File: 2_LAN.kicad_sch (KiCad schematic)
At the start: 48 parts, among them U1 LAN9514, X1 25MHz

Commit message: add LCSC part tags, silkscreen
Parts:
- C10, C9: LCSC (none) -> C1658
- C11: LCSC (none) -> C1779
- C12, C13, C14, C15, C16, C17, C18, C21, C22, C23, C24, C25, C26, C27, C28: LCSC (none) -> C14663
- C19: LCSC (none) -> C21122
- C29: LCSC (none) -> C1592
- C45, C46: LCSC (none) -> C23742
- D1: LCSC (none) -> C2687126
- F2: LCSC (none) -> C2830246
- FB1, FB2: LCSC (none) -> C14709
- LAN1: LCSC (none) -> C3021374
- R10, R12: LCSC (none) -> C25804
- R11: LCSC (none) -> C22790
- R13, R9: LCSC (none) -> C23138
- R21, R22, R23, R24, R25, R26, R27, R30: LCSC (none) -> C21189
- R6: LCSC (none) -> C22935
- R7: LCSC (none) -> C22865
- R8: LCSC (none) -> C22859
- RN1: LCSC (none) -> C136850
- U1: LCSC (none) -> C625111
- USB1, USB2: LCSC (none) -> C6386909
- X1: LCSC (none) -> C9006

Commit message: rename to x1-expander
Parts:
- C10, C9: symbol X1 Expande-easyedapro:33pF -> x1-expander:33pF
- C11: symbol X1 Expande-easyedapro:4.7uF -> x1-expander:4.7uF
- C12, C13, C14, C15, C16, C17, C18, C21, C22, C23, C24, C25, C26, C27, C28: symbol X1 Expande-easyedapro:100nF -> x1-expander:100nF
- C19: symbol X1 Expande-easyedapro:.022uF -> x1-expander:.022uF
- C29: symbol X1 Expande-easyedapro:1uF -> x1-expander:1uF
- C45, C46: symbol X1 Expande-easyedapro:75pF -> x1-expander:75pF
- D1: footprint X1 Expande-easyedapro:SOT-23-6_L2.9-W1.6-P0.95-LS2.8-BL -> x1-expander:SOT-23-6_L2.9-W1.6-P0.95-LS2.8-BL; symbol X1 Expande-easyedapro:SRV05-4.TCT_C2687126 -> x1-expander:SRV05-4.TCT_C2687126
- F2: symbol X1 Expande-easyedapro:JK-NSMD100-16V -> x1-expander:JK-NSMD100-16V
- FB1, FB2: symbol X1 Expande-easyedapro:2A/0.05DCR -> x1-expander:2A/0.05DCR
- LAN1: footprint X1 Expande-easyedapro:RJ45-TH_HC913550A-M899-A -> x1-expander:RJ45-TH_HC913550A-M899-A; symbol X1 Expande-easyedapro:HC913550A-M899-A -> x1-expander:HC913550A-M899-A
- R10, R12: symbol X1 Expande-easyedapro:10K 1/10W 1% -> x1-expander:10K 1/10W 1%
- R11: symbol X1 Expande-easyedapro:12k 1/10W 1% -> x1-expander:12k 1/10W 1%
- R13, R9: symbol X1 Expande-easyedapro:330 -> x1-expander:330
- R6: symbol X1 Expande-easyedapro:1M -> x1-expander:1M
- R7: symbol X1 Expande-easyedapro:12.4k 1% -> x1-expander:12.4k 1%
- R8: symbol X1 Expande-easyedapro:10 1/16W 1% -> x1-expander:10 1/16W 1%
- RN1: footprint X1 Expande-easyedapro:RES-ARRAY-SMD_0402-8P-L2.0-W1.0-BL -> x1-expander:RES-ARRAY-SMD_0402-8P-L2.0-W1.0-BL; symbol X1 Expande-easyedapro:49.9 -> x1-expander:49.9
- U1: footprint X1 Expande-easyedapro:QFN64G-0.5-9X9MM -> x1-expander:QFN64G-0.5-9X9MM; symbol X1 Expande-easyedapro:LAN9514 -> x1-expander:LAN9514
- USB1, USB2: footprint X1 Expande-easyedapro:USB-TH_10.0-4C6.3-ZB -> x1-expander:USB-TH_10.0-4C6.3-ZB; symbol X1 Expande-easyedapro:10.0 4C6.3 ZB -> x1-expander:10.0 4C6.3 ZB
- X1: footprint X1 Expande-easyedapro:OSC-SMD_4P-L3.2-W2.5-BL -> x1-expander:OSC-SMD_4P-L3.2-W2.5-BL; symbol X1 Expande-easyedapro:25MHz -> x1-expander:25MHz

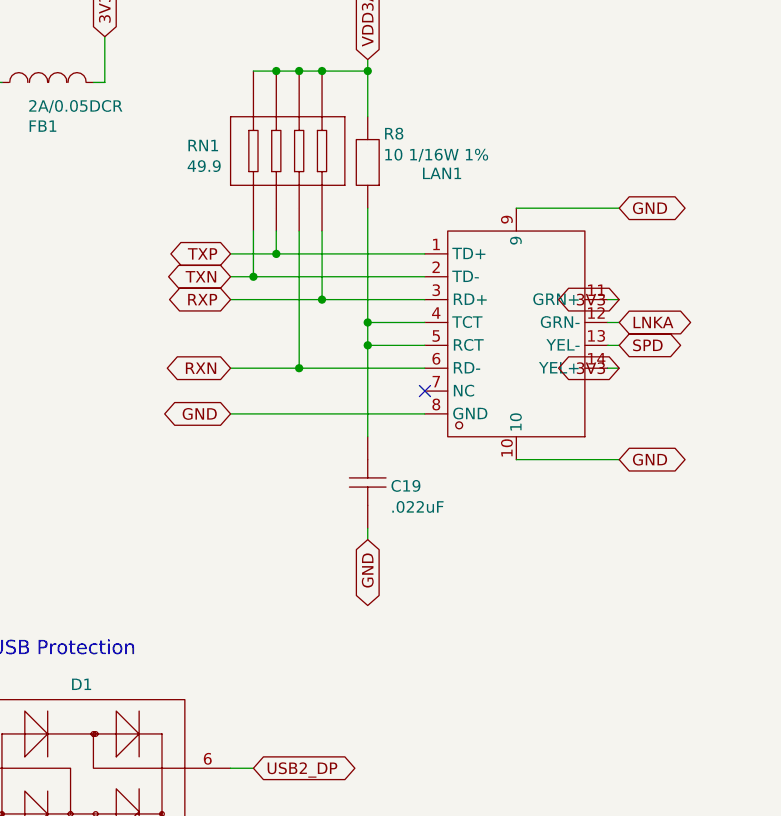
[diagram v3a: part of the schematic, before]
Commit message: replace LAN1 with C375844
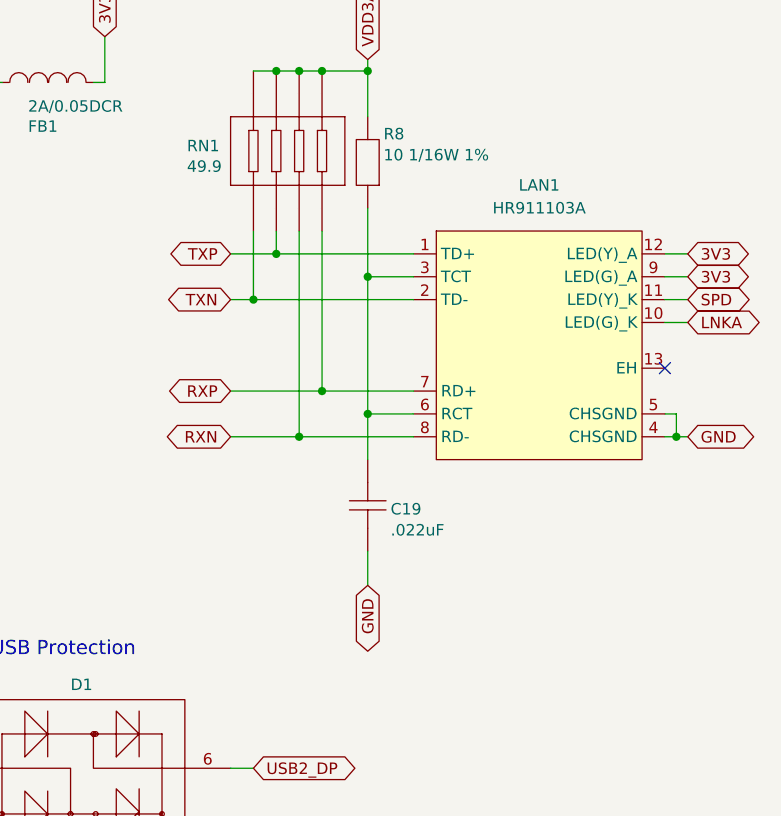
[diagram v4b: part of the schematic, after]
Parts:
- removed LAN1: HC913550A-M899-A, x1-expander:RJ45-TH_HC913550A-M899-A, symbol x1-expander:HC913550A-M899-A
- added LAN1: HR911103A, x1-expander:RJ45-TH_HR911103A, symbol x1-expander:HR911103A
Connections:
- net 3V3: now also LAN1.12 (LED(Y)_A), LAN1.9 (LED(G)_A)
- net GND: now also LAN1.4 (CHSGND), LAN1.5 (CHSGND)
- net LNKA: now also LAN1.10 (LED(G)_K)
- net RXN: now also LAN1.8 (RD-)
- net RXP: now also LAN1.7 (RD+)
- net SPD: now also LAN1.11 (LED(Y)_K)
- net TXN: now also LAN1.2 (TD-)
- net TXP: now also LAN1.1 (TD+)
- net at C19.2, R8.1: now also LAN1.3 (TCT), LAN1.6 (RCT)
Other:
- moved on the sheet: C19
